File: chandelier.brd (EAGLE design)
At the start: 74 x 29.4 mm, 18 parts, among them IC1 NDC7002N-DUAL-MOS-N, IC2 NDC7002N-DUAL-MOS-N, IC3 NDC7002N-DUAL-MOS-N, IC4 NDC7002N-DUAL-MOS-N, IC9 74595, J1 HEADER, J10 HEADER, J2 HEADER, J3 HEADER, J4 HEADER, J5 HEADER, J6 HEADER, J7 HEADER, J8 HEADER, J9 HEADER

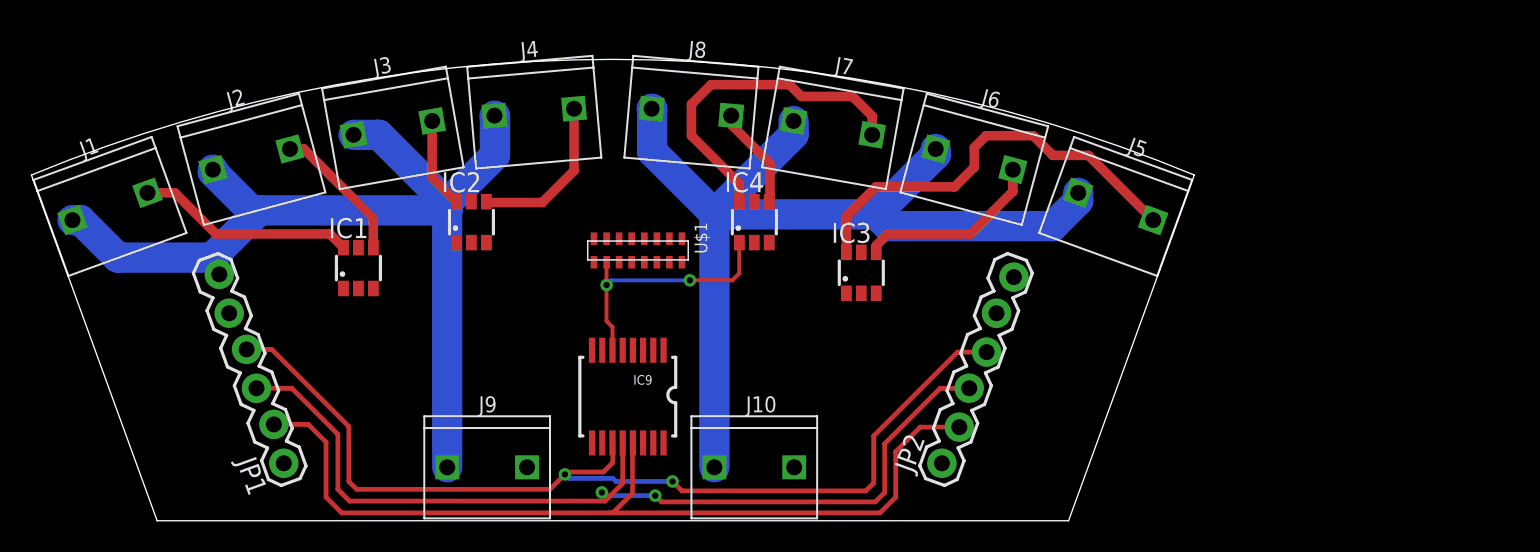
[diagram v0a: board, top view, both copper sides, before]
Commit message: adding uncommitted things
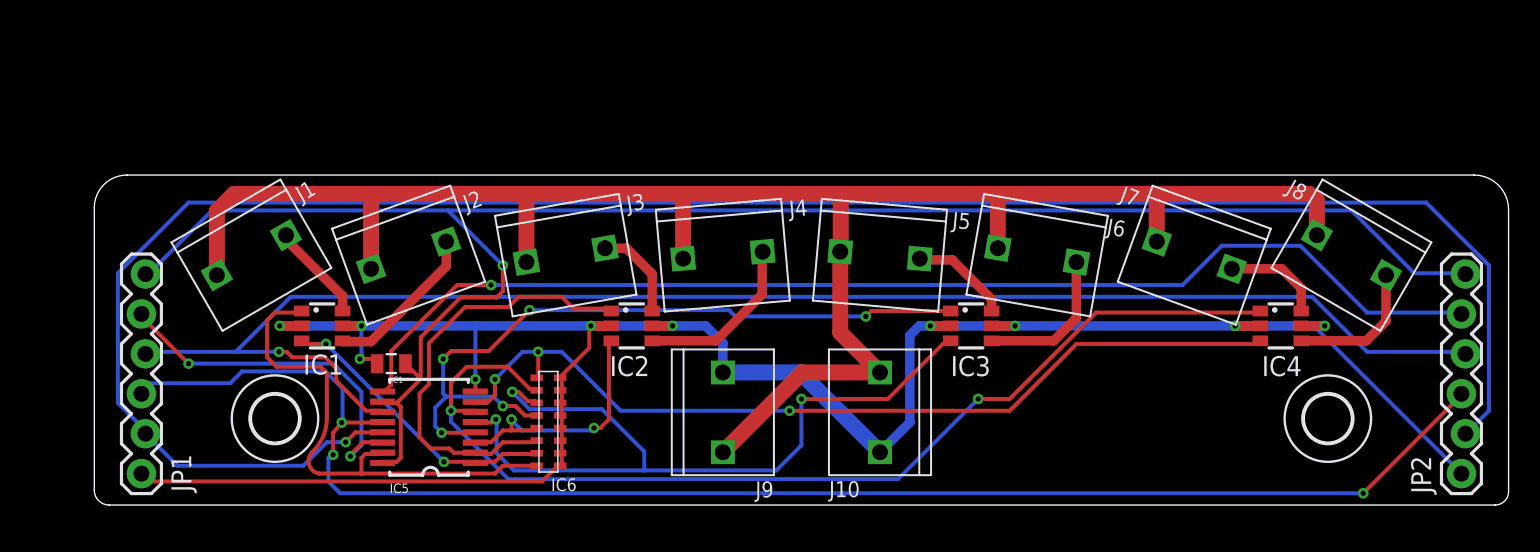
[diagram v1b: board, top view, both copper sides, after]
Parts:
- removed IC9: 74595, SparkFun-DigitalIC:TSSOP16
- removed U$1: RESISTOR-ARRAY-8, Livestream:CAY16-103J8
- added C1: 1uF, SparkFun-Capacitors:0805
- added IC5: 74595, SparkFun-DigitalIC:TSSOP16
- added IC6: RESISTOR-ARRAY-8, Livestream:CAY16-103J8
- added U$2, U$3: (no value), Livestream:HOLE-3
- moved J8 43.0 mm to (80.0, 14.9), turned to 330 degrees
- moved IC4 34.1 mm to (75.5, 10.4), turned to 270 degrees
- moved JP2 33.1 mm to (87.0, 1.00), turned to 90 degrees
- moved J7 24.4 mm to (70.0, 14.9), turned to 340 degrees
- moved J9 15.4 mm to (40.0, 4.90), turned to 90 degrees
- moved J5 15.3 mm to (50.0, 14.9), turned to 355 degrees
- moved J4 15.1 mm to (40.0, 14.9)
- moved J3 13.7 mm to (30.0, 14.9)
- moved IC2 12.1 mm to (34.2, 10.4), turned to 270 degrees
- moved J2 11.7 mm to (20.0, 14.9), turned to 20 degrees
- moved J1 9.52 mm to (10.0, 14.9), turned to 30 degrees
- moved JP1 9.08 mm to (3.00, 1.00), turned to 90 degrees
- moved J10 8.73 mm to (50.0, 4.90), turned to 270 degrees
- moved IC3 7.76 mm to (55.8, 10.4), turned to 270 degrees
- moved J6 7.29 mm to (60.0, 14.9), turned to 350 degrees
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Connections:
- removed net VCC: JP1.6, JP2.6
- net DIN: now also IC5.14; no longer IC9.14
- net DOUT: now also IC5.9; no longer IC9.9
- net G: now also IC5.13; no longer IC9.13
- net G1: now also IC5.15, IC6.2; no longer IC9.15, U$1.2
- net G2: now also IC5.1, IC6.4; no longer IC9.1, U$1.4
- net G3: now also IC5.2, IC6.6; no longer IC9.2, U$1.6
- net G4: now also IC5.3, IC6.8; no longer IC9.3, U$1.8
- net G5: now also IC5.4, IC6.10; no longer IC9.4, U$1.10
- net G6: now also IC5.5, IC6.12; no longer IC9.5, U$1.12
- net G7: now also IC5.6, IC6.14; no longer IC9.6, U$1.14
- net G8: now also IC5.7, IC6.16; no longer IC9.7, U$1.16
- net GND: now also C1.2, IC5.8, IC6.1, IC6.11, IC6.13, IC6.15, IC6.3, IC6.5, IC6.7, IC6.9; no longer IC9.8, U$1.1, U$1.11, U$1.13, U$1.15, U$1.3, U$1.5, U$1.7, U$1.9
- net RCK: now also IC5.12; no longer IC9.12
- net SCK: now also IC5.11; no longer IC9.11
- net VCC3V3: now also C1.1, IC5.10, IC5.16, JP1.6, JP2.6; no longer IC9.10, IC9.16
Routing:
- net GND: track 0.00 -> 147.0 mm, vias 0 -> 10
- net VCC3V3: track 0.00 -> 112.4 mm, vias 0 -> 1
- net DOUT: track 0.00 -> 75.6 mm, vias 0 -> 1
- net G: track 56.9 -> 129.9 mm, vias 0 -> 1
- net G8: track 0.00 -> 57.0 mm, vias 0 -> 3
- net G7: track 16.5 -> 68.0 mm
- net G6: track 0.00 -> 51.2 mm, vias 0 -> 3
- net G5: track 0.00 -> 47.5 mm, vias 0 -> 5
- net RCK: track 60.5 -> 97.9 mm, vias 2 -> 3
- net SCK: track 63.7 -> 98.5 mm, vias 2 -> 1
- net G1: track 0.00 -> 32.1 mm
- net G3: track 0.00 -> 27.7 mm
- net DIN: track 0.00 -> 23.3 mm, vias 0 -> 2
- net N$5: track 26.9 -> 6.39 mm
- net G2: track 0.00 -> 18.5 mm, vias 0 -> 2
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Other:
- board size 74 x 29.4 mm -> 90 x 21 mm
